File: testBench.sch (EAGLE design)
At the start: 29 parts, among them IC1 NCS21911SN2T1G, IC2 NCS21911SN2T1G, IC3 NCS21911SN2T1G, IC4 NCS21911SN2T1G, IC5 NCS21911SN2T1G

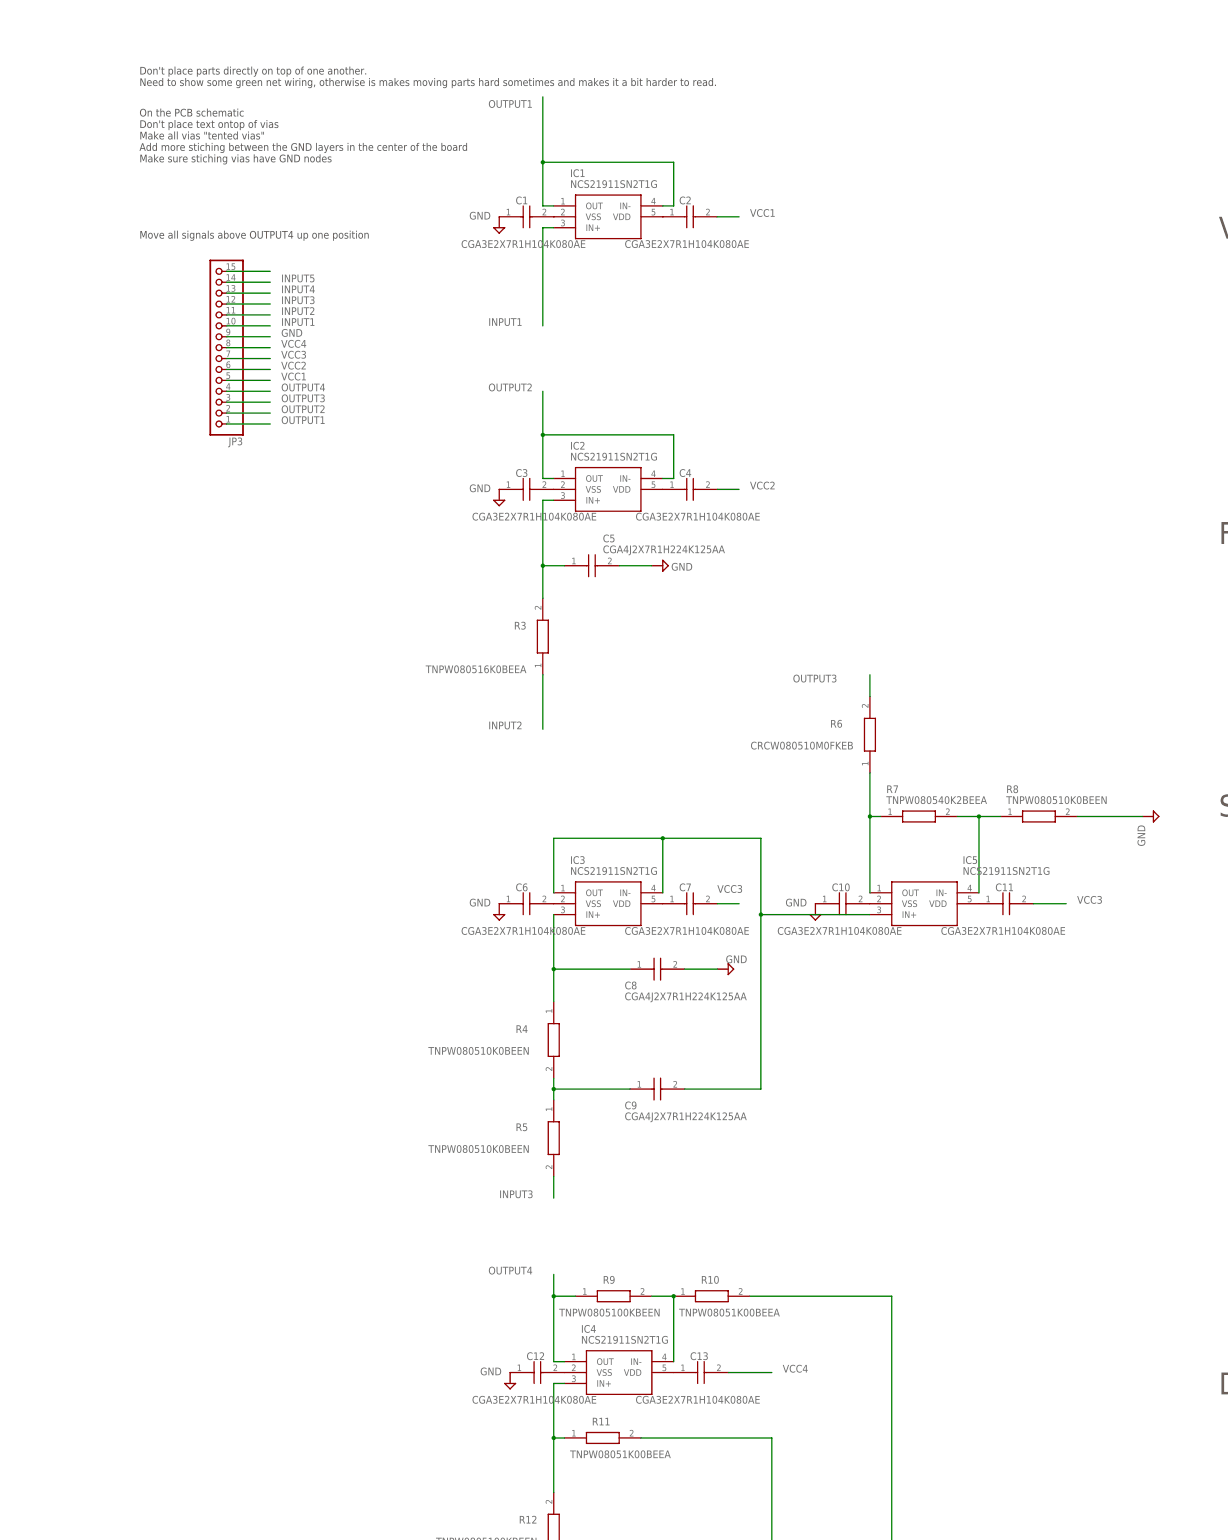
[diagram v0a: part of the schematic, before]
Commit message: This is my third PCB for opamp test bench
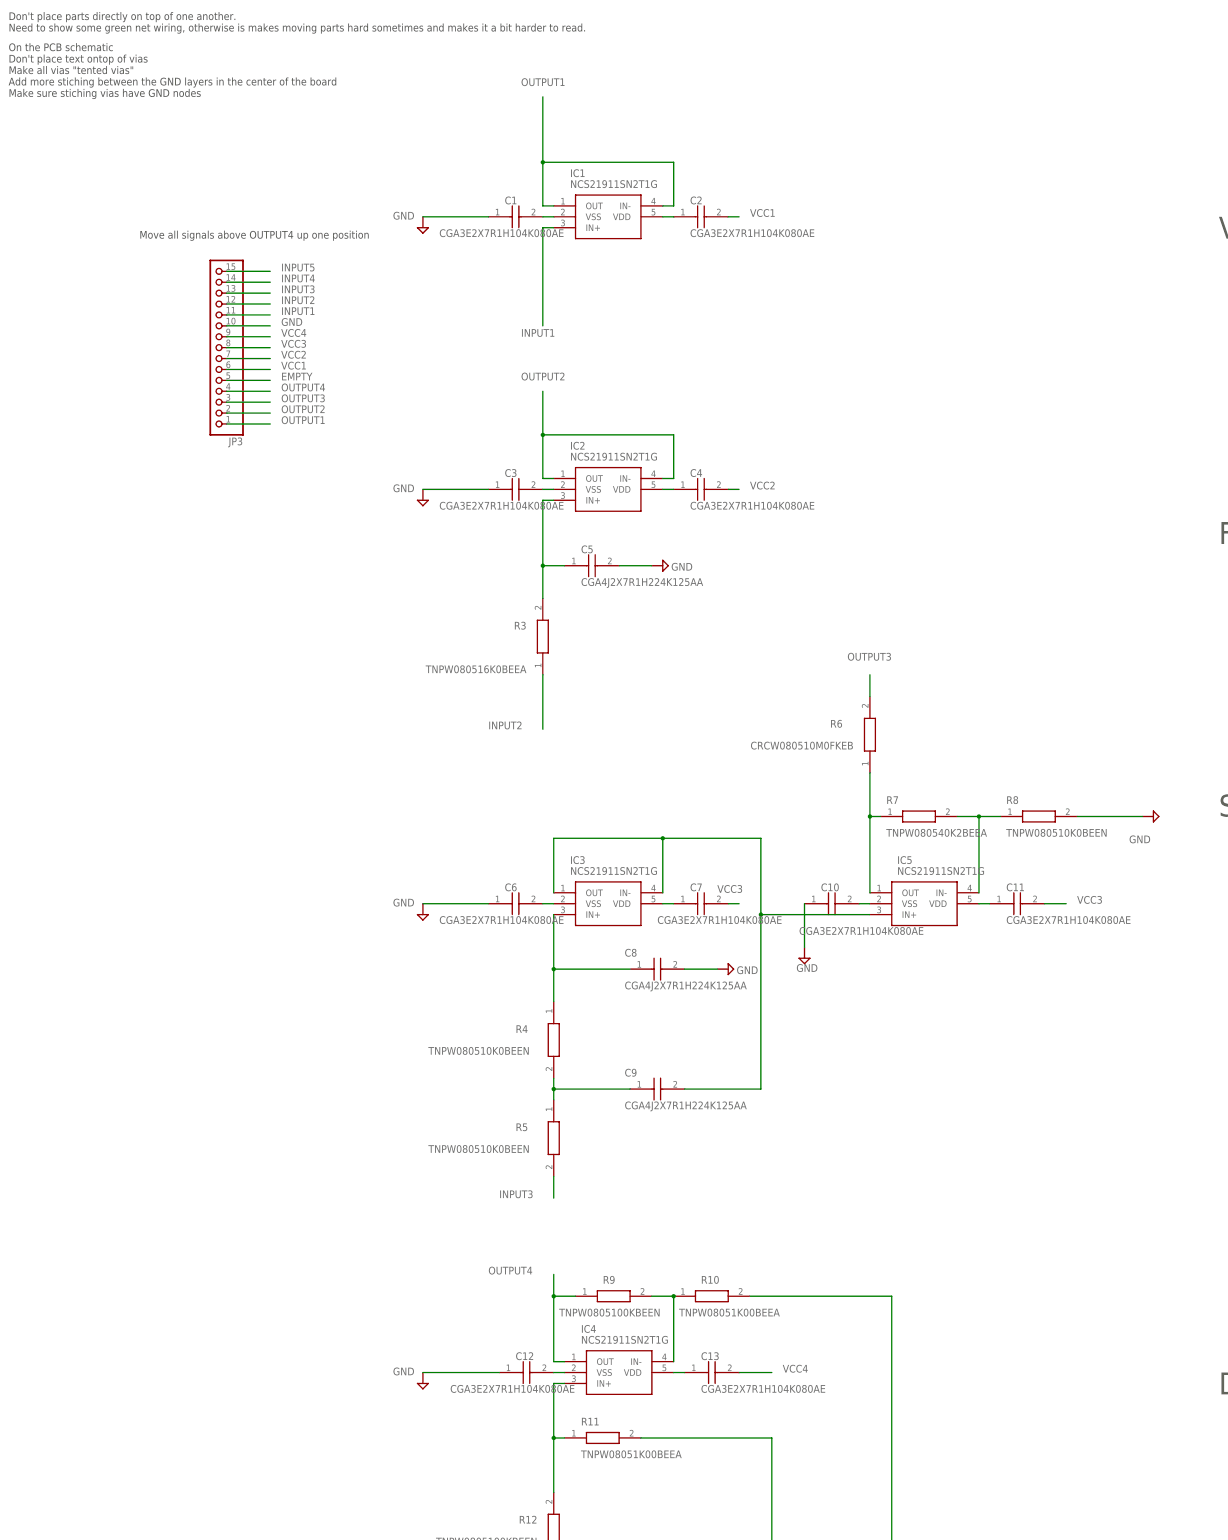
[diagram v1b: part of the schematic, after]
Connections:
- removed net N$44: JP3.15
- new net EMPTY: JP3.5
- net GND: now also JP3.10; no longer JP3.9
- net INPUT1: now also JP3.11; no longer JP3.10
- net INPUT2: now also JP3.12; no longer JP3.11
- net INPUT3: now also JP3.13; no longer JP3.12
- net INPUT4: now also JP3.14; no longer JP3.13
- net INPUT5: now also JP3.15; no longer JP3.14
- net VCC1: now also JP3.6; no longer JP3.5
- net VCC2: now also JP3.7; no longer JP3.6
- net VCC3: now also JP3.8; no longer JP3.7
- net VCC4: now also JP3.9; no longer JP3.8
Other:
- moved on the sheet: C1, C10, C11, C12, C13, C2, C3, C4, C6, C7

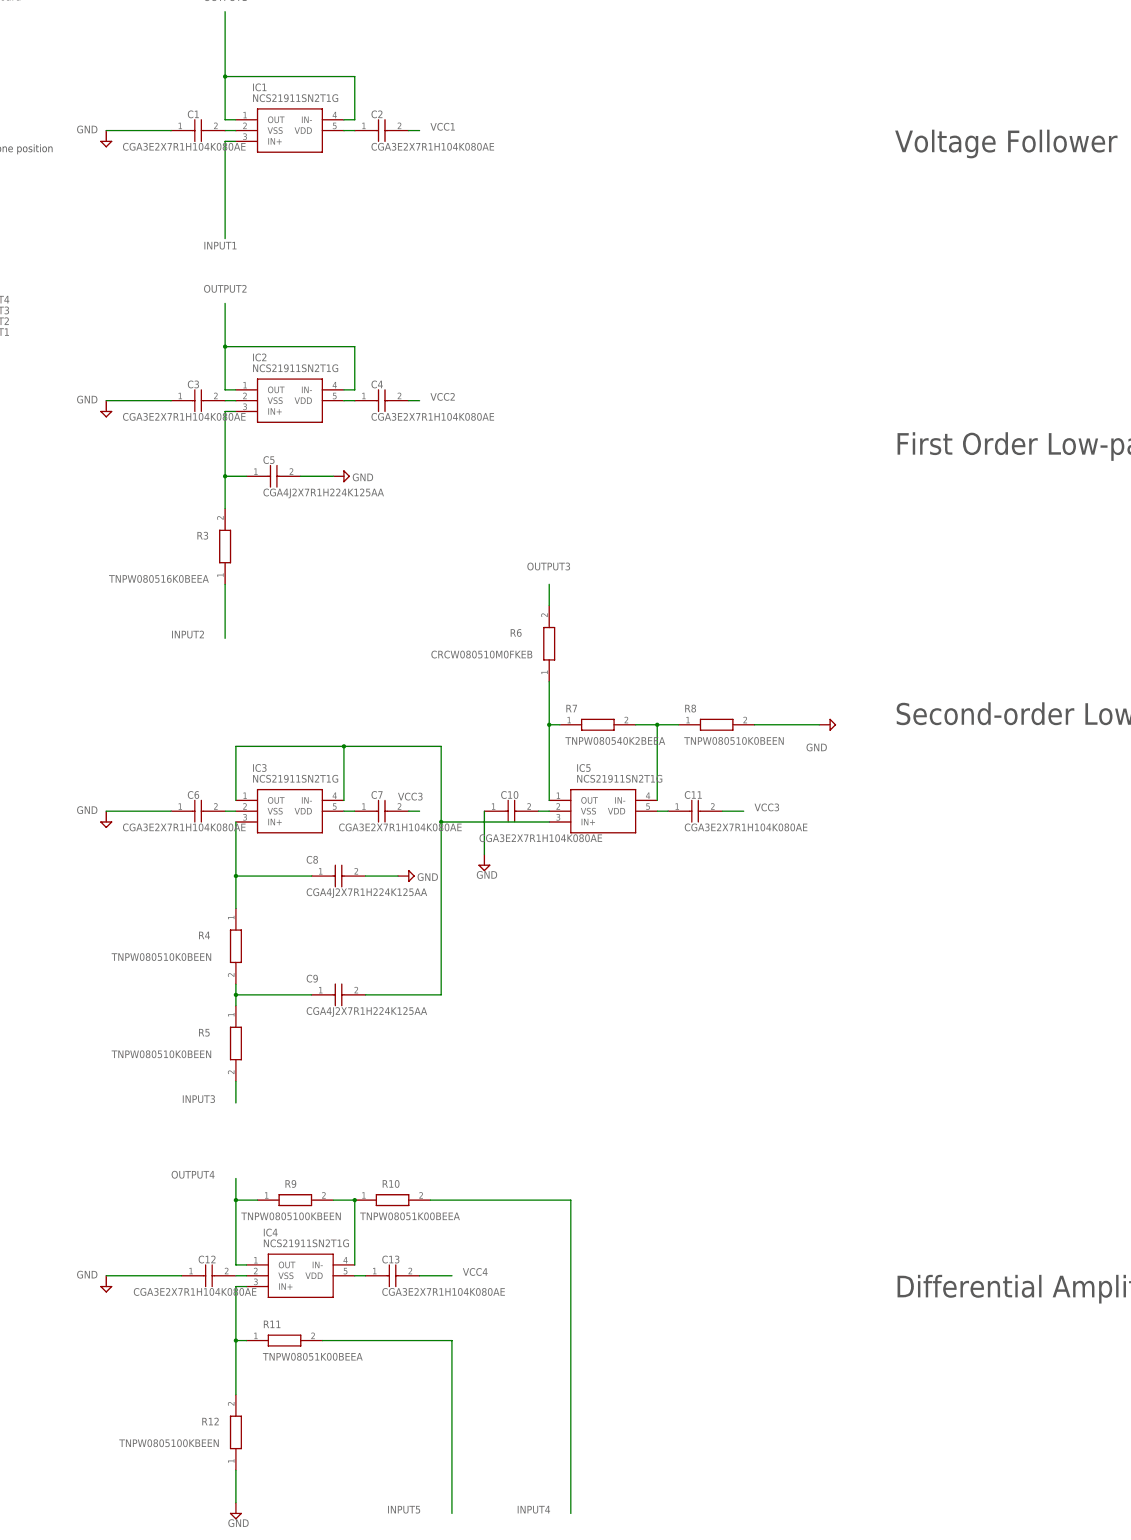
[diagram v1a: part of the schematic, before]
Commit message: PCB test bench fourth version
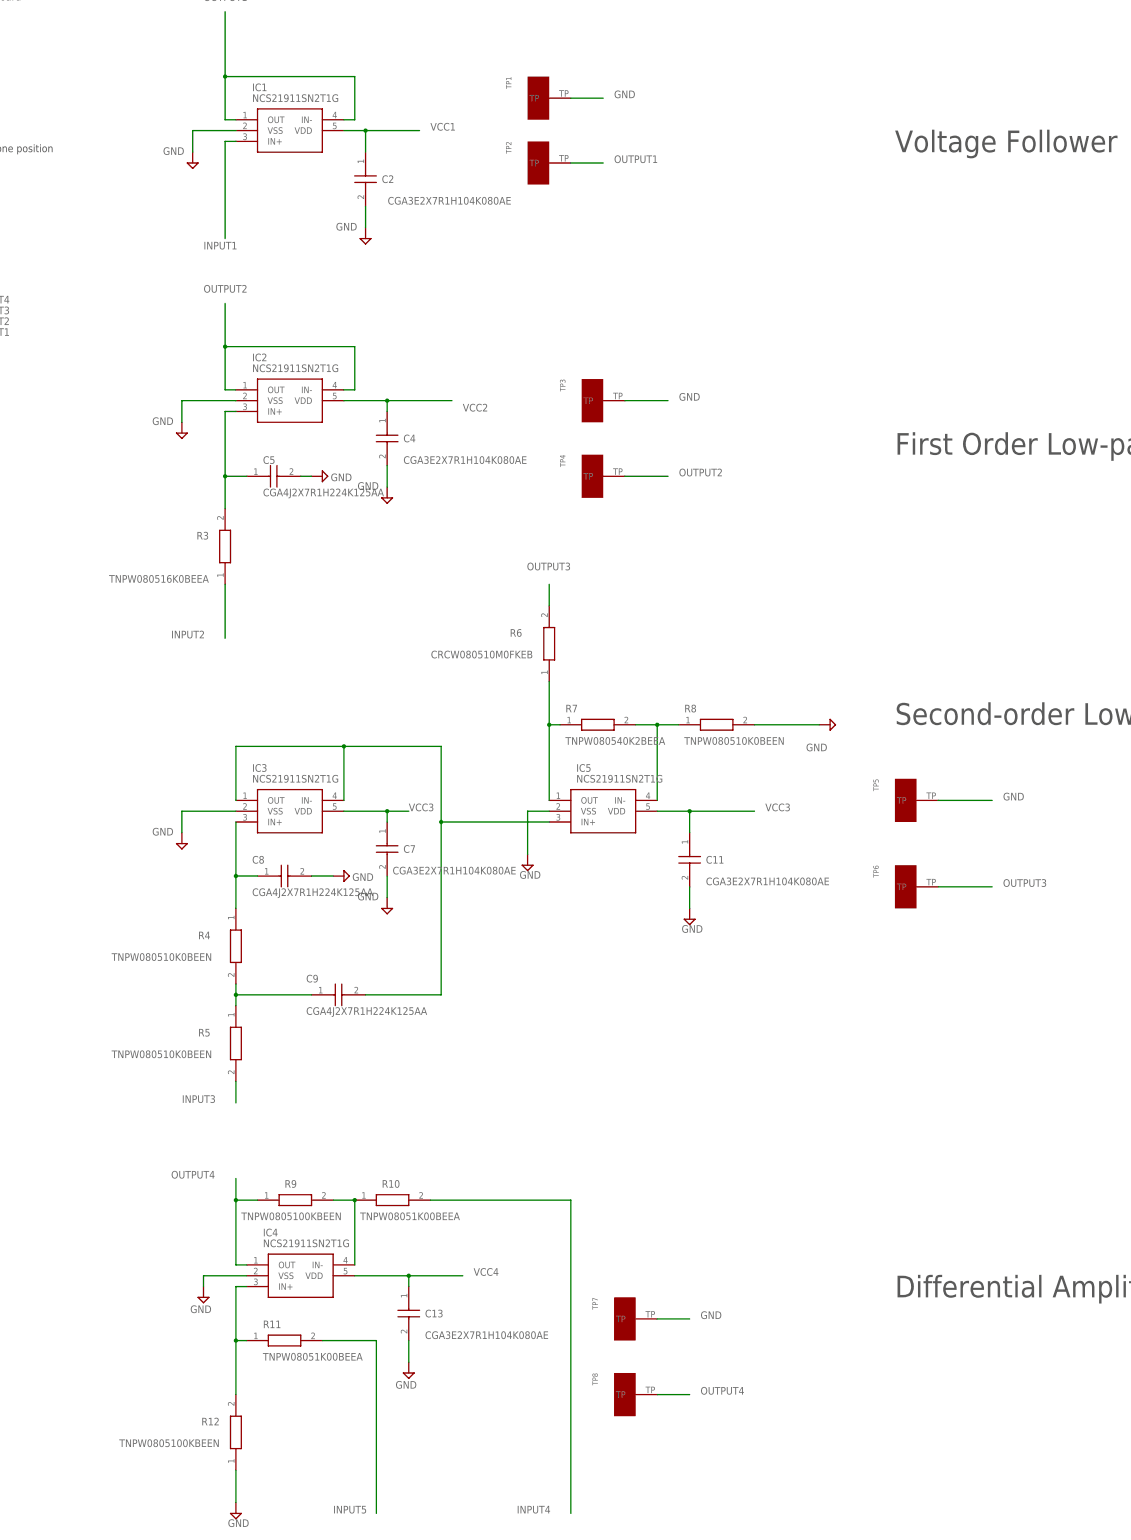
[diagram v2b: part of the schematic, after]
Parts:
- removed C1, C10, C12, C3, C6: CGA3E2X7R1H104K080AE, SamacSys_Parts:CGA3E2X7R1H104K080AE
- added TP1, TP2, TP3, TP4, TP5, TP6, TP7, TP8: (no value), SamacSys_Parts:S1751-46R
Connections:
- removed net N$16: C11.1, IC5.VDD
- removed net N$17: C10.2, IC5.VSS
- removed net N$2: C1.2, IC1.VSS
- removed net N$3: C2.1, IC1.VDD
- removed net N$4: C3.2, IC2.VSS
- removed net N$5: C4.1, IC2.VDD
- removed net N$6: C6.2, IC3.VSS
- removed net N$7: C7.1, IC3.VDD
- removed net N$8: C13.1, IC4.VDD
- removed net N$9: C12.2, IC4.VSS
- net GND: now also C11.2, C13.2, C2.2, C4.2, C7.2, IC1.VSS, IC2.VSS, IC3.VSS, IC4.VSS, IC5.VSS, TP1.TP, TP3.TP, TP5.TP, TP7.TP; no longer C1.1, C10.1, C12.1, C3.1, C6.1
- net OUTPUT1: now also TP2.TP
- net OUTPUT2: now also TP4.TP
- net OUTPUT3: now also TP6.TP
- net OUTPUT4: now also TP8.TP
- net VCC1: now also C2.1, IC1.VDD; no longer C2.2
- net VCC2: now also C4.1, IC2.VDD; no longer C4.2
- net VCC3: now also C11.1, C7.1, IC3.VDD, IC5.VDD; no longer C11.2, C7.2
- net VCC4: now also C13.1, IC4.VDD; no longer C13.2
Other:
- moved on the sheet: C11, C13, C2, C4, C7, C8

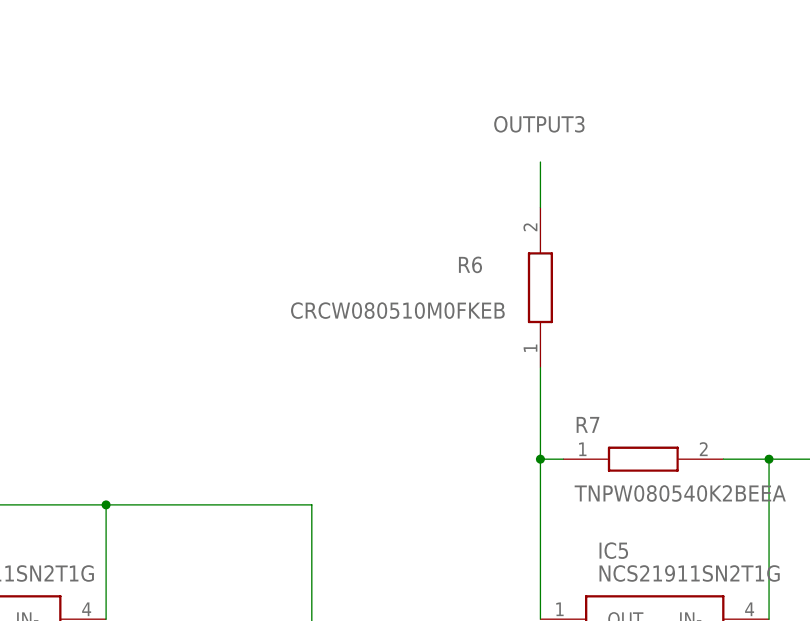
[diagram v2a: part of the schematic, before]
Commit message: pcb test bench 6th version
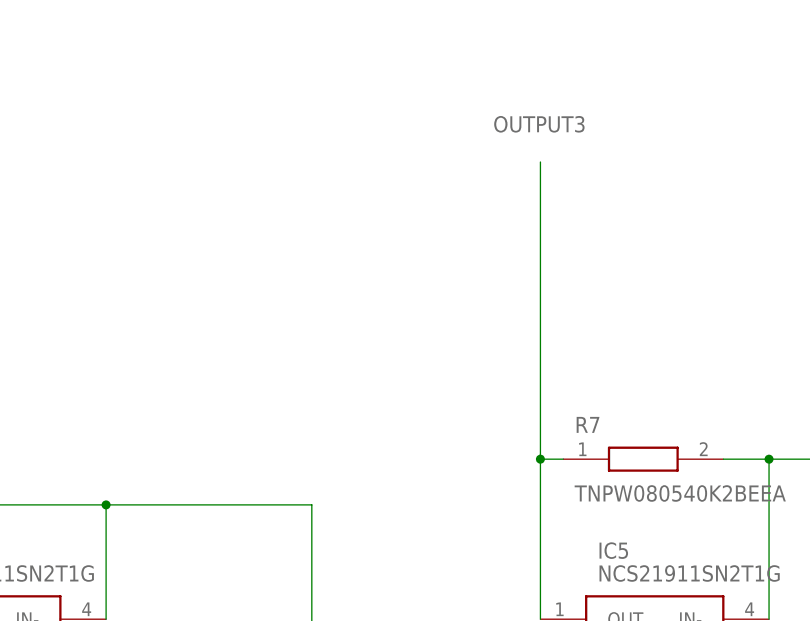
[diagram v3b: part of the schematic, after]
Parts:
- removed R6: CRCW080510M0FKEB, SamacSys_Parts:CRCW080510M0FKEB
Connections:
- removed net N$18: IC5.OUT, R6.1, R7.1
- net OUTPUT3: now also IC5.OUT, R7.1; no longer R6.2
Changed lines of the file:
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@@
 <part name="C11" library="SamacSys_Parts" deviceset="CGA3E2X7R1H104K080AE" device=""/>
 <part name="SUPPLY10" library="supply2" library_urn="urn:adsk.eagle:library:372" deviceset="GND" device=""/>
-<part name="R6" library="SamacSys_Parts" deviceset="CRCW080510M0FKEB" device=""/>
 <part name="SUPPLY13" library="supply2" library_urn="urn:adsk.eagle:library:372" deviceset="GND" device=""/>
 <part name="R8" library="SamacSys_Parts" deviceset="TNPW080510K0BEEN" device=""/>
@@
 <attribute name="VALUE" x="36.195" y="-140.335" size="1.778" layer="96"/>
 </instance>
-<instance part="R6" gate="G$1" x="43.18" y="-93.98" smashed="yes" rot="R90">
-<attribute name="NAME" x="36.83" y="-82.55" size="1.778" layer="95" rot="R180" align="center-left"/>
-<attribute name="VALUE" x="39.37" y="-87.63" size="1.778" layer="96" rot="R180" align="center-left"/>
-</instance>
 <instance part="SUPPLY13" gate="GND" x="-5.08" y="-139.7" smashed="yes" rot="R90">
 <attribute name="VALUE" x="1.905" y="-139.065" size="1.778" layer="96" rot="R180"/>
@@
 </segment>
 </net>
-<net name="N$18" class="0">
-<segment>
+<net name="OUTPUT3" class="0">
+<segment>
+<label x="48.26" y="-66.04" size="1.778" layer="95" rot="R180"/>
 <pinref part="IC5" gate="G$1" pin="OUT"/>
-<pinref part="R6" gate="G$1" pin="1"/>
 <wire x1="43.18" y1="-121.92" x2="43.18" y2="-104.14" width="0.1524" layer="91"/>
 <pinref part="R7" gate="G$1" pin="1"/>
-<wire x1="43.18" y1="-104.14" x2="43.18" y2="-93.98" width="0.1524" layer="91"/>
 <wire x1="43.18" y1="-104.14" x2="45.72" y2="-104.14" width="0.1524" layer="91"/>
 <junction x="43.18" y="-104.14"/>
-</segment>
-</net>
-<net name="OUTPUT3" class="0">
-<segment>
-<pinref part="R6" gate="G$1" pin="2"/>
-<wire x1="43.18" y1="-76.2" x2="43.18" y2="-71.12" width="0.1524" layer="91"/>
-<label x="48.26" y="-66.04" size="1.778" layer="95" rot="R180"/>
-</segment>
-<segment>
+<wire x1="43.18" y1="-71.12" x2="43.18" y2="-104.14" width="0.1524" layer="91"/>
+</segment>
+<segment>
